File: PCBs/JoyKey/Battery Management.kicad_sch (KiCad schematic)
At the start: 17 parts, among them J4 JST PH, Q1 PMOS,Si7157DP, U1 BQ25060, U4 LP2981-3.3

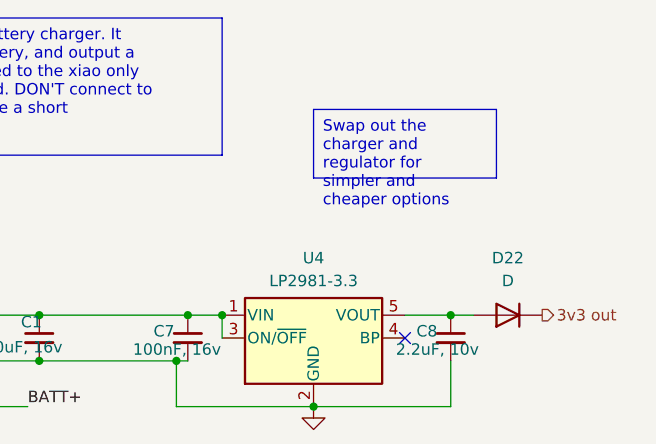
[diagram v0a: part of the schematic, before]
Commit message: Assigned footprints for batt management
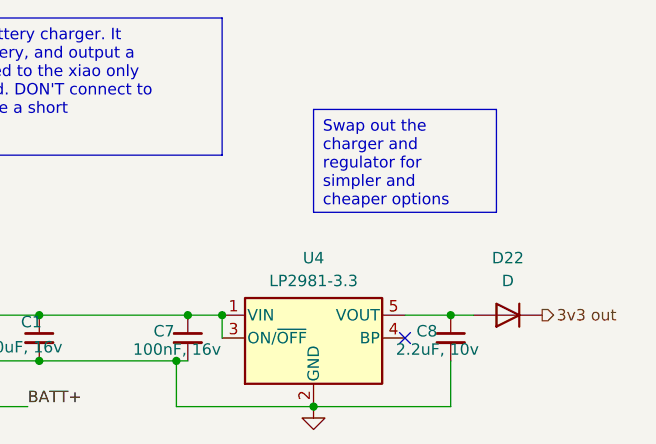
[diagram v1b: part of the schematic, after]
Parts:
- D22: footprint (none) -> Diode_SMD:D_0805_2012Metric
- J4: footprint (none) -> Connector_JST:JST_PH_S2B-PH-SM4-TB_1x02-1MP_P2.00mm_Horizontal
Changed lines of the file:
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@@
 		(exclude_from_sim no)
 		(at 180.34 83.82 0)
-		(size 20.32 7.62)
+		(size 20.32 11.43)
 		(stroke
 			(width 0)
@@
 			)
 		)
-		(property "Footprint" ""
+		(property "Footprint" "Connector_JST:JST_PH_S2B-PH-SM4-TB_1x02-1MP_P2.00mm_Horizontal"
 			(at 189.23 147.32 0)
 			(effects
@@
 			)
 		)
-		(property "Footprint" ""
+		(property "Footprint" "Diode_SMD:D_0805_2012Metric"
 			(at 201.93 106.68 0)
 			(effects
